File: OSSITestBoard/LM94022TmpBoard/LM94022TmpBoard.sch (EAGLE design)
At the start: 8 parts, among them U1 LM94022, X1 P-PAD-S, X2 P-PAD-S, X3 P-PAD-S

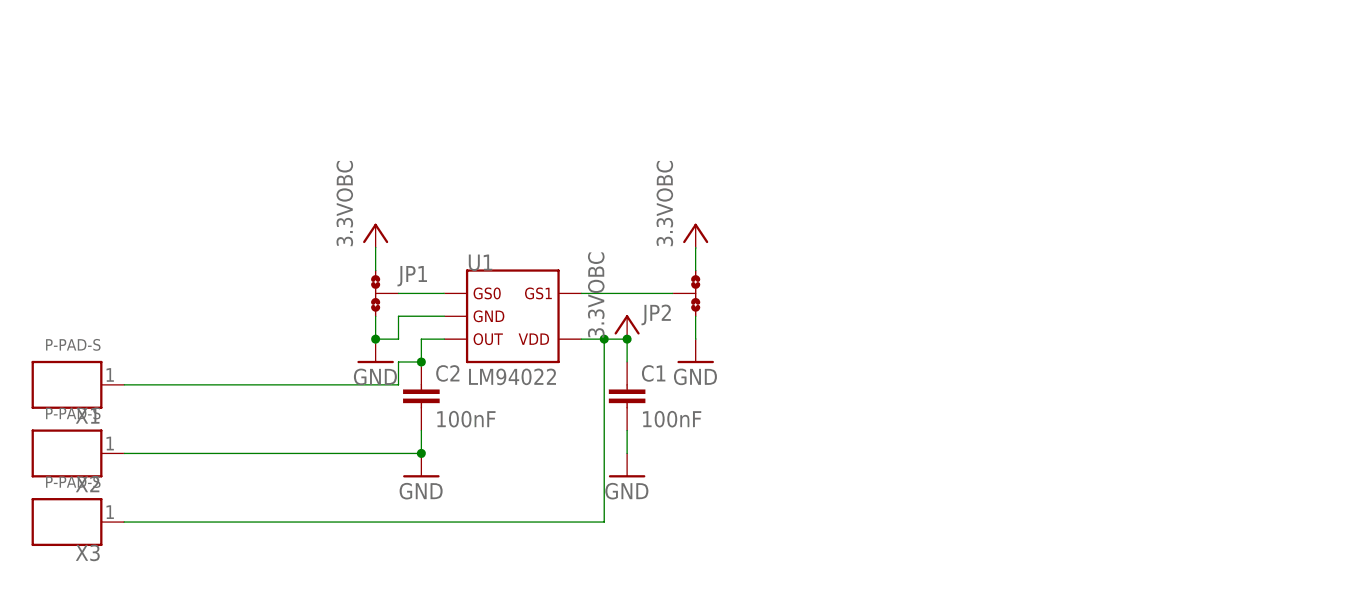
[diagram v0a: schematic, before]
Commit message: comment added
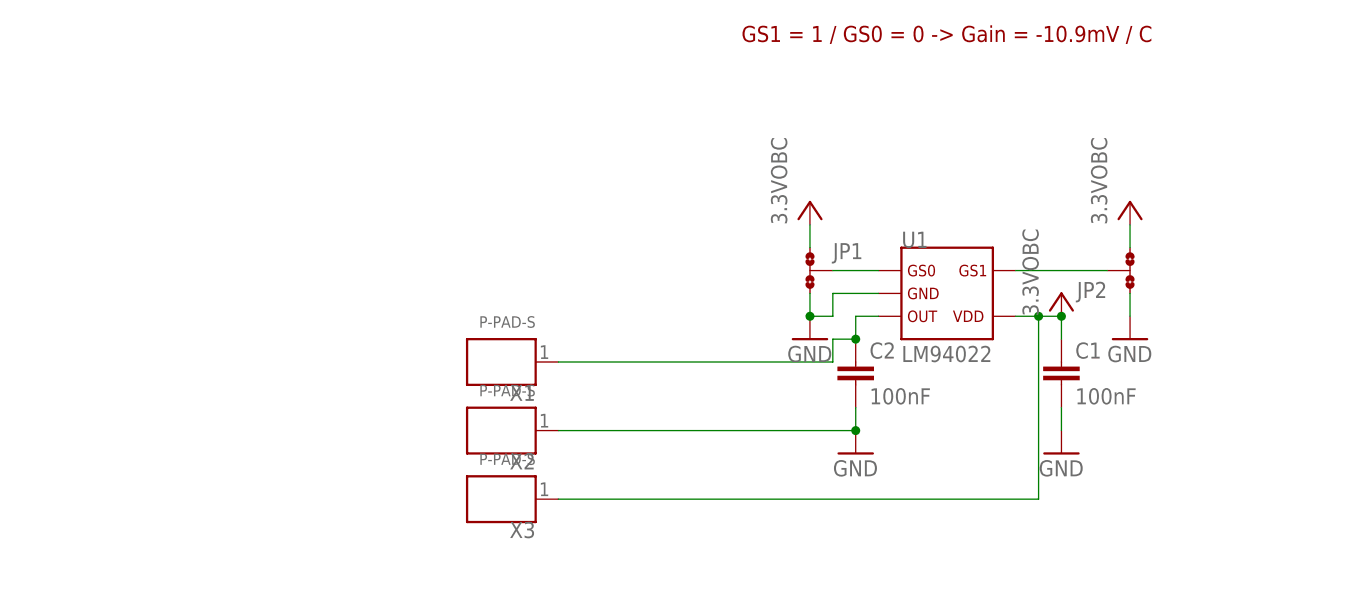
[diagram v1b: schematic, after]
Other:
- note added: "GS1 = 1 / GS0 = 0 -> Gain = -10.9mV / C"
- moved on the sheet: C1, C2, JP1, JP2, U1, X1, X2, X3
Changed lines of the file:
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@@
 <sheet>
 <plain>
+<text x="104.14" y="124.46" size="1.778" layer="94">GS1 = 1 / GS0 = 0 -&gt; Gain = -10.9mV / C</text>
 </plain>
 <instances>
 <instance part="FRAME1" gate="G$1" x="0" y="0"/>
 <instance part="FRAME1" gate="G$2" x="162.56" y="0"/>
-<instance part="U1" gate="G$1" x="78.74" y="93.98"/>
-<instance part="C1" gate="G$1" x="91.44" y="86.36"/>
-<instance part="GND3" gate="1" x="91.44" y="76.2"/>
-<instance part="JP1" gate="G$1" x="63.5" y="96.52"/>
-<instance part="JP2" gate="G$1" x="99.06" y="96.52" rot="R180"/>
-<instance part="3.3VOBC4" gate="G$1" x="99.06" y="101.6"/>
-<instance part="GND6" gate="1" x="99.06" y="88.9"/>
-<instance part="3.3VOBC5" gate="G$1" x="91.44" y="91.44"/>
-<instance part="GND7" gate="1" x="63.5" y="88.9"/>
-<instance part="3.3VOBC1" gate="G$1" x="63.5" y="101.6"/>
-<instance part="C2" gate="G$1" x="68.58" y="86.36"/>
-<instance part="GND1" gate="1" x="68.58" y="76.2"/>
-<instance part="X1" gate="G$1" x="30.48" y="86.36" rot="R180"/>
-<instance part="X2" gate="G$1" x="30.48" y="78.74" rot="R180"/>
-<instance part="X3" gate="G$1" x="30.48" y="71.12" rot="R180"/>
+<instance part="U1" gate="G$1" x="127" y="96.52"/>
+<instance part="C1" gate="G$1" x="139.7" y="88.9"/>
+<instance part="GND3" gate="1" x="139.7" y="78.74"/>
+<instance part="JP1" gate="G$1" x="111.76" y="99.06"/>
+<instance part="JP2" gate="G$1" x="147.32" y="99.06" rot="R180"/>
+<instance part="3.3VOBC4" gate="G$1" x="147.32" y="104.14"/>
+<instance part="GND6" gate="1" x="147.32" y="91.44"/>
+<instance part="3.3VOBC5" gate="G$1" x="139.7" y="93.98"/>
+<instance part="GND7" gate="1" x="111.76" y="91.44"/>
+<instance part="3.3VOBC1" gate="G$1" x="111.76" y="104.14"/>
+<instance part="C2" gate="G$1" x="116.84" y="88.9"/>
+<instance part="GND1" gate="1" x="116.84" y="78.74"/>
+<instance part="X1" gate="G$1" x="78.74" y="88.9" rot="R180"/>
+<instance part="X2" gate="G$1" x="78.74" y="81.28" rot="R180"/>
+<instance part="X3" gate="G$1" x="78.74" y="73.66" rot="R180"/>
 </instances>
 <busses>
@@
 <pinref part="GND3" gate="1" pin="GND"/>
 <pinref part="C1" gate="G$1" pin="2"/>
-<wire x1="91.44" y1="78.74" x2="91.44" y2="81.28" width="0.1524" layer="91"/>
+<wire x1="139.7" y1="81.28" x2="139.7" y2="83.82" width="0.1524" layer="91"/>
 </segment>
 <segment>
 <pinref part="GND6" gate="1" pin="GND"/>
 <pinref part="JP2" gate="G$1" pin="1"/>
-<wire x1="99.06" y1="91.44" x2="99.06" y2="93.98" width="0.1524" layer="91"/>
+<wire x1="147.32" y1="93.98" x2="147.32" y2="96.52" width="0.1524" layer="91"/>
 </segment>
 <segment>
 <pinref part="JP1" gate="G$1" pin="3"/>
 <pinref part="GND7" gate="1" pin="GND"/>
-<wire x1="63.5" y1="91.44" x2="63.5" y2="93.98" width="0.1524" layer="91"/>
+<wire x1="111.76" y1="93.98" x2="111.76" y2="96.52" width="0.1524" layer="91"/>
 <pinref part="U1" gate="G$1" pin="P$2"/>
-<wire x1="71.12" y1="93.98" x2="66.04" y2="93.98" width="0.1524" layer="91"/>
-<wire x1="66.04" y1="93.98" x2="66.04" y2="91.44" width="0.1524" layer="91"/>
-<wire x1="66.04" y1="91.44" x2="63.5" y2="91.44" width="0.1524" layer="91"/>
-<junction x="63.5" y="91.44"/>
+<wire x1="119.38" y1="96.52" x2="114.3" y2="96.52" width="0.1524" layer="91"/>
+<wire x1="114.3" y1="96.52" x2="114.3" y2="93.98" width="0.1524" layer="91"/>
+<wire x1="114.3" y1="93.98" x2="111.76" y2="93.98" width="0.1524" layer="91"/>
+<junction x="111.76" y="93.98"/>
 </segment>
 <segment>
 <pinref part="GND1" gate="1" pin="GND"/>
 <pinref part="C2" gate="G$1" pin="2"/>
-<wire x1="68.58" y1="78.74" x2="68.58" y2="81.28" width="0.1524" layer="91"/>
+<wire x1="116.84" y1="81.28" x2="116.84" y2="83.82" width="0.1524" layer="91"/>
 <pinref part="X2" gate="G$1" pin="P$1"/>
-<wire x1="35.56" y1="78.74" x2="68.58" y2="78.74" width="0.1524" layer="91"/>
-<junction x="68.58" y="78.74"/>
+<wire x1="83.82" y1="81.28" x2="116.84" y2="81.28" width="0.1524" layer="91"/>
+<junction x="116.84" y="81.28"/>
 </segment>
 </net>
@@
 <pinref part="U1" gate="G$1" pin="P$4"/>
 <pinref part="C1" gate="G$1" pin="1"/>
-<wire x1="86.36" y1="91.44" x2="88.9" y2="91.44" width="0.1524" layer="91"/>
-<wire x1="88.9" y1="91.44" x2="91.44" y2="91.44" width="0.1524" layer="91"/>
-<wire x1="91.44" y1="91.44" x2="91.44" y2="88.9" width="0.1524" layer="91"/>
+<wire x1="134.62" y1="93.98" x2="137.16" y2="93.98" width="0.1524" layer="91"/>
+<wire x1="137.16" y1="93.98" x2="139.7" y2="93.98" width="0.1524" layer="91"/>
+<wire x1="139.7" y1="93.98" x2="139.7" y2="91.44" width="0.1524" layer="91"/>
 <pinref part="3.3VOBC5" gate="G$1" pin="3.3VOBC"/>
-<junction x="91.44" y="91.44"/>
+<junction x="139.7" y="93.98"/>
 <pinref part="X3" gate="G$1" pin="P$1"/>
-<wire x1="35.56" y1="71.12" x2="88.9" y2="71.12" width="0.1524" layer="91"/>
-<wire x1="88.9" y1="71.12" x2="88.9" y2="91.44" width="0.1524" layer="91"/>
-<junction x="88.9" y="91.44"/>
+<wire x1="83.82" y1="73.66" x2="137.16" y2="73.66" width="0.1524" layer="91"/>
+<wire x1="137.16" y1="73.66" x2="137.16" y2="93.98" width="0.1524" layer="91"/>
+<junction x="137.16" y="93.98"/>
 </segment>
 <segment>
 <pinref part="JP2" gate="G$1" pin="3"/>
 <pinref part="3.3VOBC4" gate="G$1" pin="3.3VOBC"/>
-<wire x1="99.06" y1="99.06" x2="99.06" y2="101.6" width="0.1524" layer="91"/>
+<wire x1="147.32" y1="101.6" x2="147.32" y2="104.14" width="0.1524" layer="91"/>
 </segment>
 <segment>
 <pinref part="JP1" gate="G$1" pin="1"/>
 <pinref part="3.3VOBC1" gate="G$1" pin="3.3VOBC"/>
-<wire x1="63.5" y1="99.06" x2="63.5" y2="101.6" width="0.1524" layer="91"/>
+<wire x1="111.76" y1="101.6" x2="111.76" y2="104.14" width="0.1524" layer="91"/>
 </segment>
 </net>
@@
 <pinref part="U1" gate="G$1" pin="P$5"/>
 <pinref part="JP2" gate="G$1" pin="2"/>
-<wire x1="86.36" y1="96.52" x2="96.52" y2="96.52" width="0.1524" layer="91"/>
+<wire x1="134.62" y1="99.06" x2="144.78" y2="99.06" width="0.1524" layer="91"/>
 </segment>
 </net>
@@
 <pinref part="U1" gate="G$1" pin="P$1"/>
 <pinref part="JP1" gate="G$1" pin="2"/>
-<wire x1="71.12" y1="96.52" x2="66.04" y2="96.52" width="0.1524" layer="91"/>
+<wire x1="119.38" y1="99.06" x2="114.3" y2="99.06" width="0.1524" layer="91"/>
 </segment>
 </net>
@@
 <segment>
 <pinref part="U1" gate="G$1" pin="P$3"/>
-<wire x1="71.12" y1="91.44" x2="68.58" y2="91.44" width="0.1524" layer="91"/>
-<wire x1="68.58" y1="91.44" x2="68.58" y2="88.9" width="0.1524" layer="91"/>
+<wire x1="119.38" y1="93.98" x2="116.84" y2="93.98" width="0.1524" layer="91"/>
+<wire x1="116.84" y1="93.98" x2="116.84" y2="91.44" width="0.1524" layer="91"/>
 <pinref part="C2" gate="G$1" pin="1"/>
 <pinref part="X1" gate="G$1" pin="P$1"/>
-<wire x1="35.56" y1="86.36" x2="66.04" y2="86.36" width="0.1524" layer="91"/>
-<wire x1="66.04" y1="86.36" x2="66.04" y2="88.9" width="0.1524" layer="91"/>
-<wire x1="66.04" y1="88.9" x2="68.58" y2="88.9" width="0.1524" layer="91"/>
-<junction x="68.58" y="88.9"/>
+<wire x1="83.82" y1="88.9" x2="114.3" y2="88.9" width="0.1524" layer="91"/>
+<wire x1="114.3" y1="88.9" x2="114.3" y2="91.44" width="0.1524" layer="91"/>
+<wire x1="114.3" y1="91.44" x2="116.84" y2="91.44" width="0.1524" layer="91"/>
+<junction x="116.84" y="91.44"/>
 </segment>
 </net>
